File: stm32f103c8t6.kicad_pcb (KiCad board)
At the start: 2 copper layers, 23.8 x 32.5 mm, 33 parts, among them IC1 AS5600-ASOT, J1 USB4105GFA, J2 SWD_Debugger, J4 DUMMY_PINS, U1 STM32F103C8T6, U2 AMS1117-3.3, Y1 Crystal

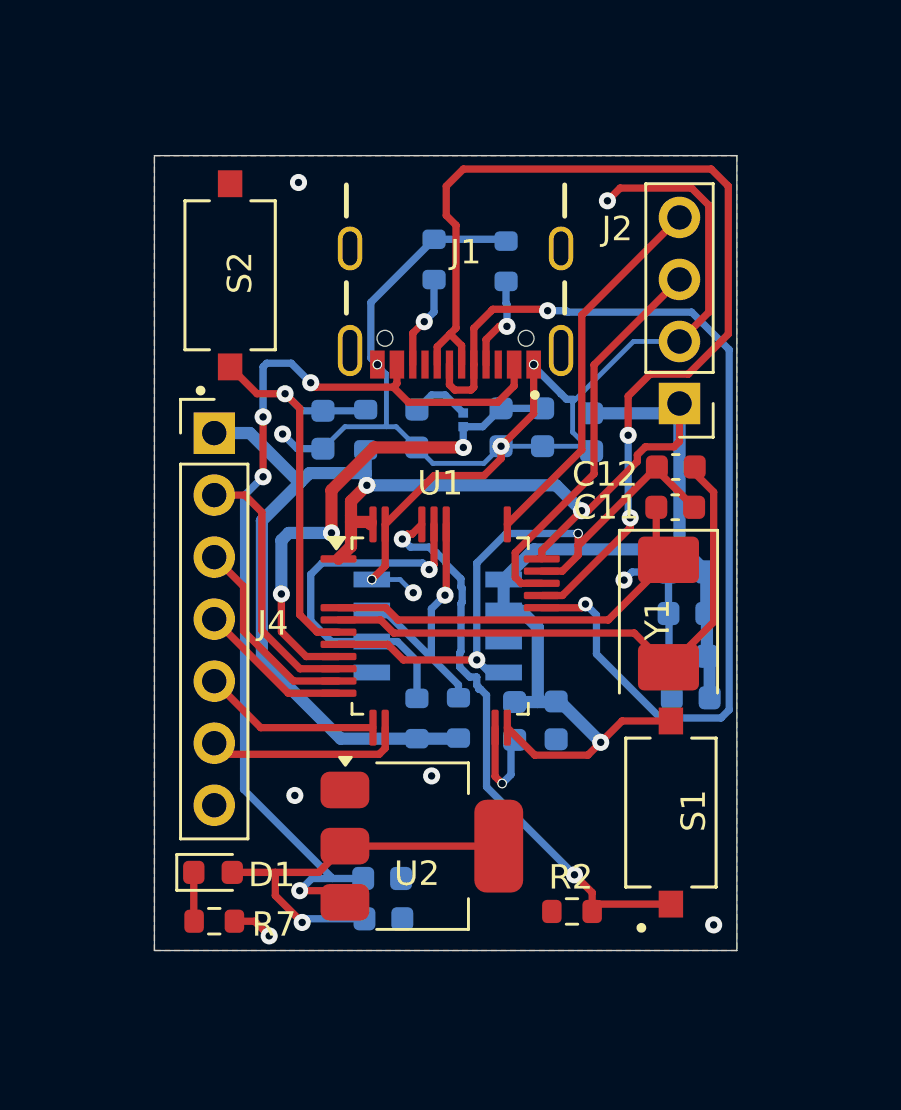
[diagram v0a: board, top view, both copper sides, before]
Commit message: Add files via upload
final pcb with mounting holes before DFM check
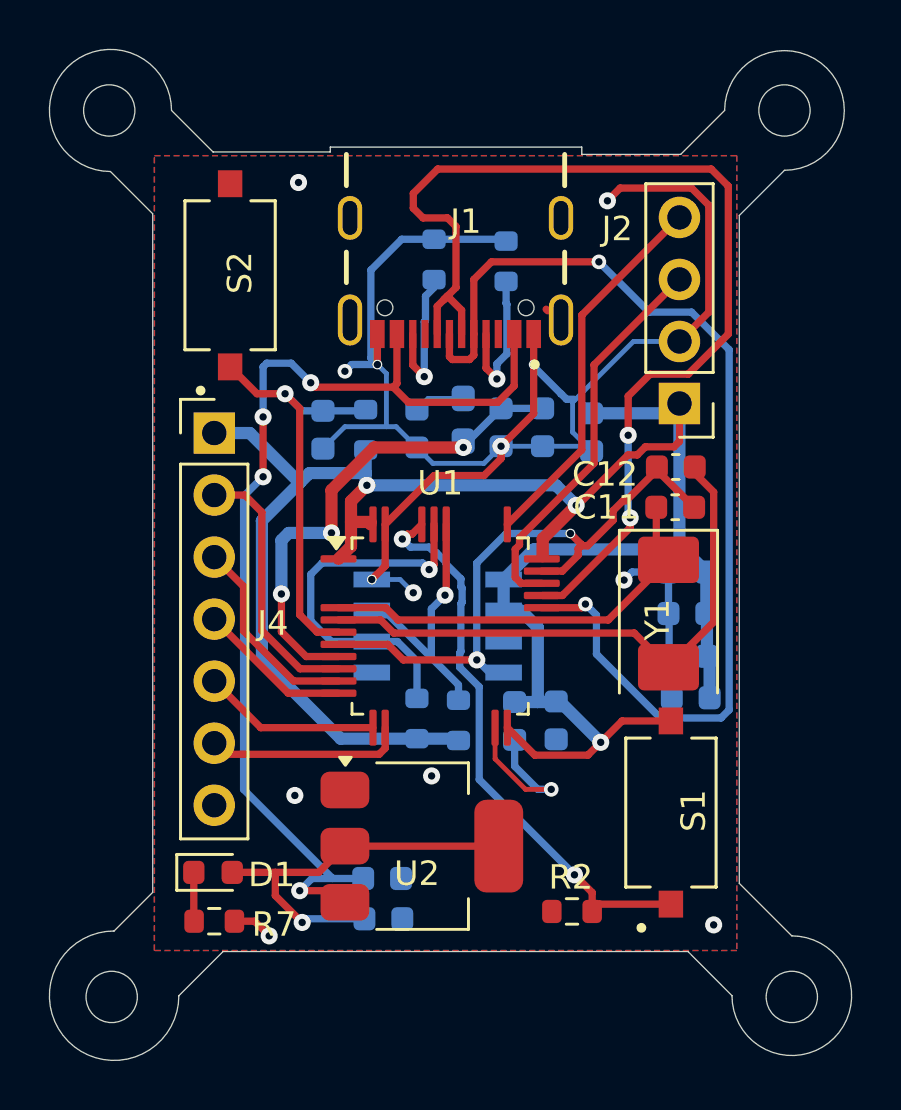
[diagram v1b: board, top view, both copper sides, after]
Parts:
- added H1: MountingHole, MountingHole:MountingHole_2.1mm, F.Cu at (134.4, 58.1)
- added H2: MountingHole, MountingHole:MountingHole_2.1mm, F.Cu at (162.1, 58.1)
- added H3: MountingHole, MountingHole:MountingHole_2.1mm, F.Cu at (134.6, 94.4)
- added H4: MountingHole, MountingHole:MountingHole_2.1mm, F.Cu at (162.4, 94.4)
- 120R1: footprint ferrite_bead:BEADC0603X33N -> Inductor_SMD:L_0603_1608Metric_Pad1.05x0.95mm_HandSolder
- moved J1 1.25 mm to (148.6, 62.5)
- moved R3 0.10 mm to (148.8, 83.1)
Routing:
- net GND: track 100.3 -> 106.0 mm
- net VBUS: track 40.8 -> 43.3 mm
- net Net-(J1-CC1): track 3.96 -> 6.24 mm
- net Net-(J1-CC2): track 3.84 -> 6.11 mm
- net /USB_D+: track 42.8 -> 44.4 mm
- net /USB_D-: track 41.3 -> 42.9 mm
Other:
- board size 23.8 x 32.5 mm -> 32.8 x 41.4 mm
